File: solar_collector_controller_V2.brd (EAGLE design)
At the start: 49.5 x 50 mm, 31 parts, among them IC1 REG1117, J1 POWER_JACKSLT, T1 BC337, X1 GND D2 VCC, X2 GND D9 VCC, X3 GND A3 VCC, X4 VCC A4 A5 GND, X5 GND A1 A2 VCC, X6 A7 A6

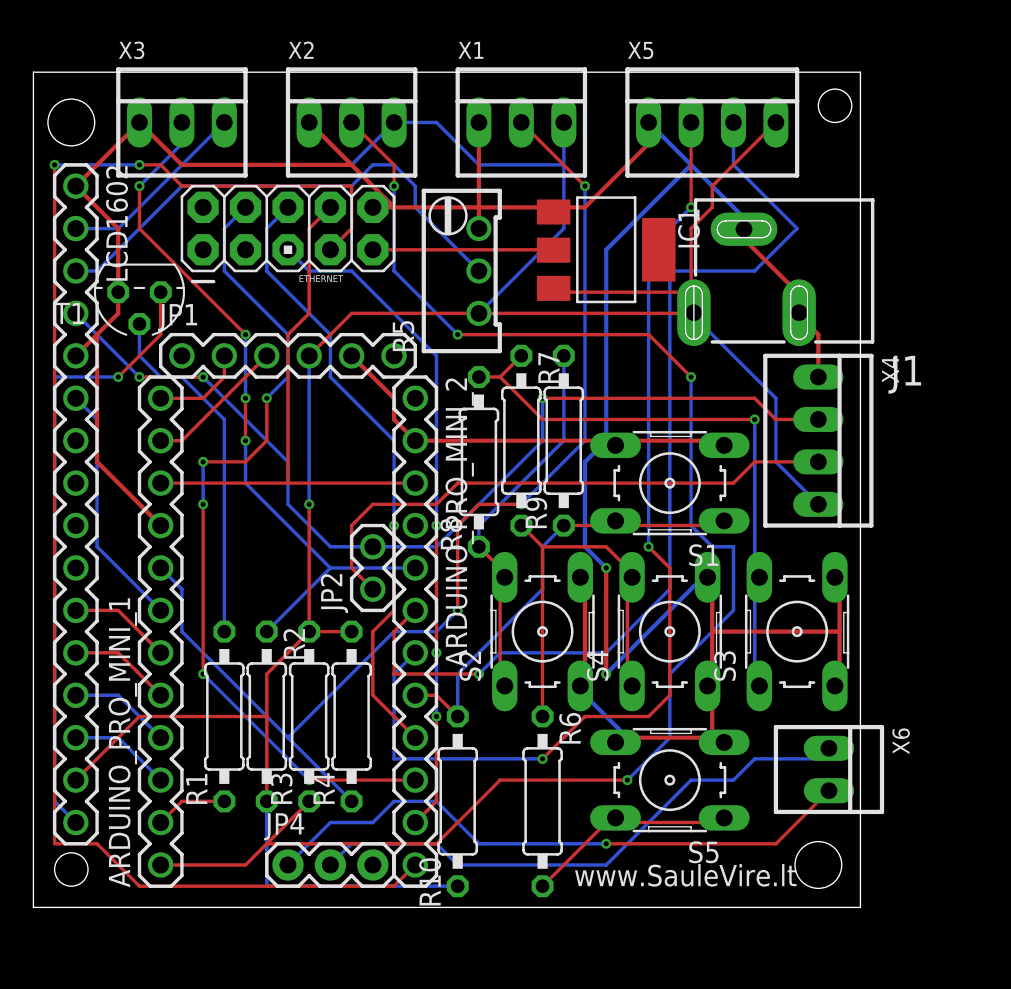
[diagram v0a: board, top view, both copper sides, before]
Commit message: pastumdyta detalės...
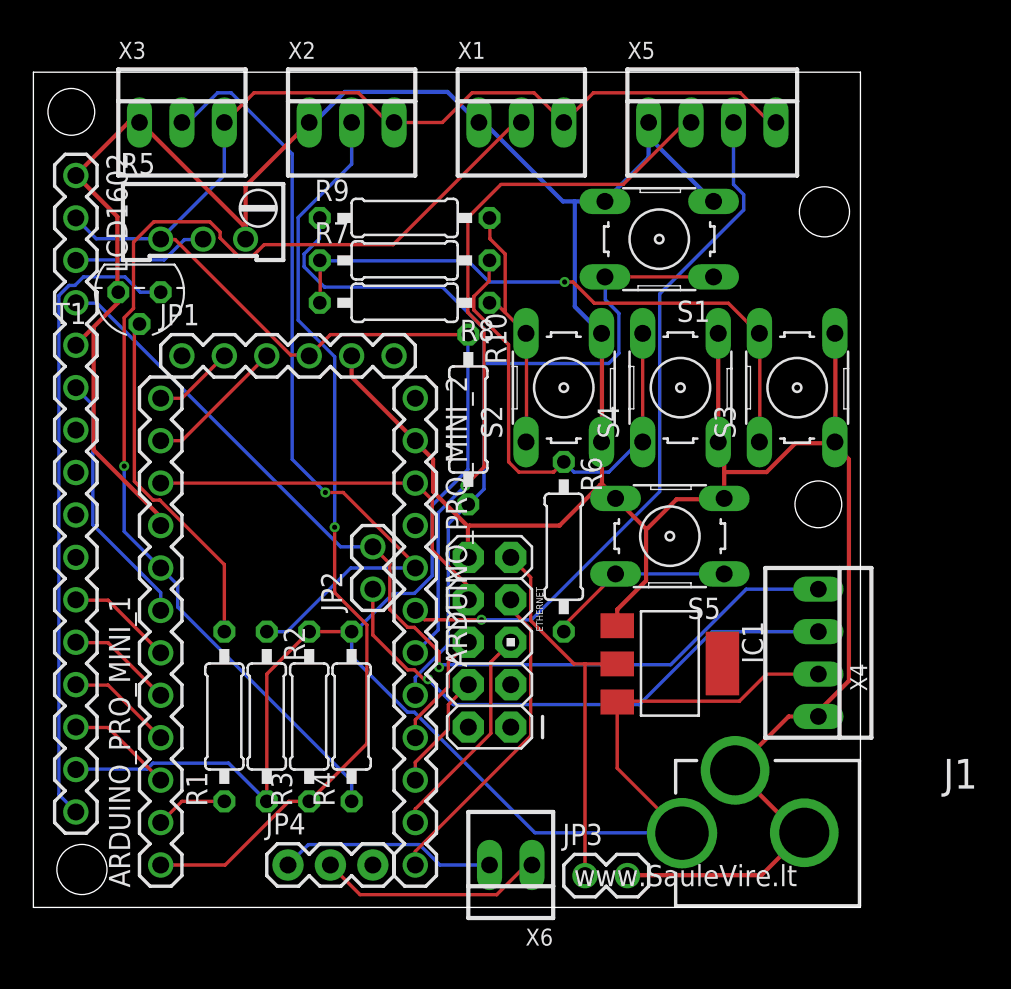
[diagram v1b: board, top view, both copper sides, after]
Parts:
- added JP3: (no value), SparkFun:1X02
- J1: value POWER_JACKSLT -> POWER; device SparkFun-Connectors:POWER_JACK_SLOT -> SparkFun-Connectors:POWER_JACK_PTH_LOCK
- moved J1 28.6 mm to (52.7, 4.45)
- moved ETHERNET 27.5 mm to (27.3, 15.9), turned to 180 degrees
- moved IC1 25.1 mm to (38.1, 14.6)
- moved R10 22.9 mm to (26.0, 29.2), turned to 90 degrees
- moved X6 19.9 mm to (28.6, 2.54), turned to 180 degrees
- moved R9 16.4 mm to (22.2, 41.3), turned to 180 degrees
- moved R5 15.6 mm to (10.2, 41.3), turned to 270 degrees
- moved R6 15.3 mm to (31.8, 21.6)
- moved S2 14.7 mm to (31.8, 31.1)
- moved S1 14.6 mm to (37.5, 40.0)
- moved S4 14.6 mm to (38.7, 31.1)
- moved S5 14.6 mm to (38.1, 22.2)
- moved S3 14.6 mm to (45.7, 31.1)
- moved R7 12.9 mm to (22.2, 38.7), turned to 180 degrees
- moved X4 12.7 mm to (47.0, 15.2)
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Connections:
- net 3.3V: now also JP3.1
- net A4: now also X4.2; no longer X4.3
- net A5: now also X4.1; no longer X4.2
- net GND: now also J1.GND, J1.GNDBREAK, JP3.2, X4.4; no longer J1.GND@1, J1.GND@2, X4.1
- net VCC: now also X4.3; no longer X4.4
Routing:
- net D10: track 86.5 -> 19.2 mm, vias 2 -> 0
- net D12: track 49.0 -> 7.03 mm, vias 5 -> 0
- net D9: track 92.5 -> 55.6 mm, vias 4 -> 1
- net A0: track 26.9 -> 59.1 mm
- net D13: track 37.0 -> 7.03 mm, vias 1 -> 0
- net D11: track 40.0 -> 13.2 mm, vias 3 -> 0
- net A7: track 36.3 -> 13.1 mm, vias 1 -> 0
- net N$1: track 30.1 -> 8.18 mm
- net A6: track 33.8 -> 13.5 mm
- net A1: track 60.8 -> 43.9 mm, vias 3 -> 1
- net A2: track 58.6 -> 42.5 mm
- net 3.3V: track 10.8 -> 23.2 mm
- net RESET: track 32.8 -> 23.5 mm
- net GND: track 211.5 -> 204.2 mm, vias 2 -> 0
- net N$11: track 22.6 -> 15.5 mm
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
